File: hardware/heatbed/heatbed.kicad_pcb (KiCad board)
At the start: 2 copper layers, 80 x 80 mm, 8 parts, among them J1 Conn_01x01, J2 Conn_01x01

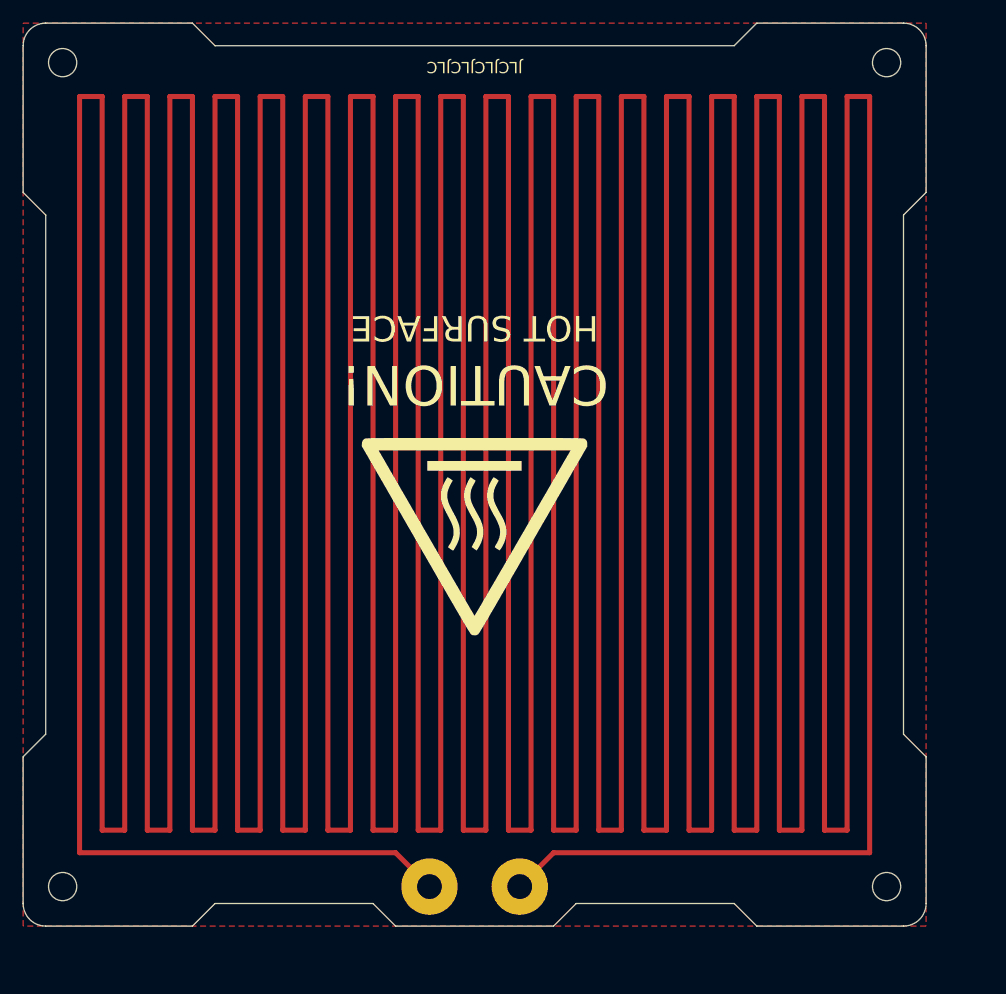
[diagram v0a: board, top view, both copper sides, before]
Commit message: Remove mounting hole silkscreen circles
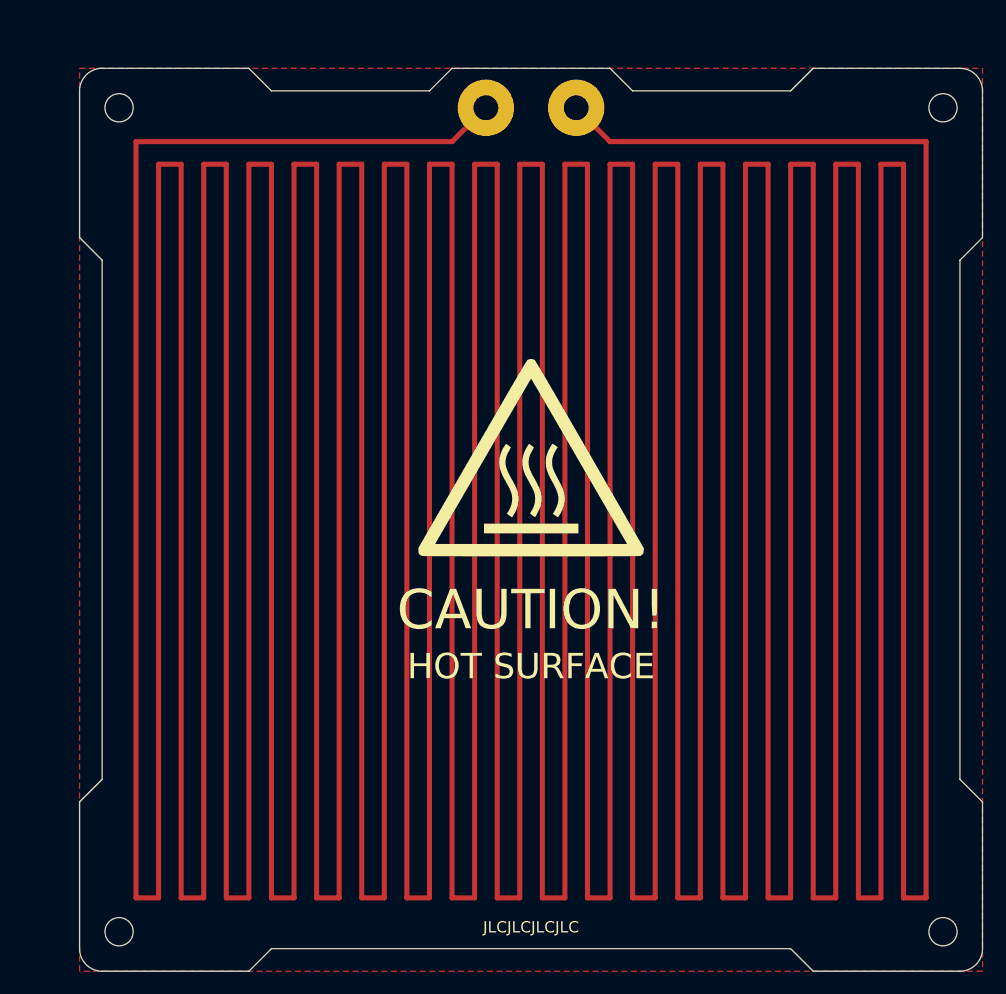
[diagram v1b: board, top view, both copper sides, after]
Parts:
- H1, H2, H3, H4: footprint Local_Library:MountingHole_2.5mm -> MountingHole:MountingHole_2.5mm
- moved H4 109.6 mm to (184.5, 136.5), turned to 180 degrees
- moved H1 104.1 mm to (184.5, 63.5), turned to 180 degrees
- moved H3 102.7 mm to (111.5, 136.5), turned to 180 degrees
- moved H2 96.9 mm to (111.5, 63.5), turned to 180 degrees
- moved J1 70.2 mm to (152.0, 63.5), turned to 180 degrees
- moved J2 69.1 mm to (144.0, 63.5), turned to 180 degrees
- moved G*** 8.60 mm to (148.0, 94.5), turned to 0 degrees
- moved G*** 8.60 mm to (148.0, 94.5), turned to 180 degrees
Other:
- outline, holes or cut-outs redrawn
